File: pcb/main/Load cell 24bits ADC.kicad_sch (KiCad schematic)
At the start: 17 parts, among them J9 SJ, Q4 TRANSISTOR_PNPMMBT4403, U4 HX711

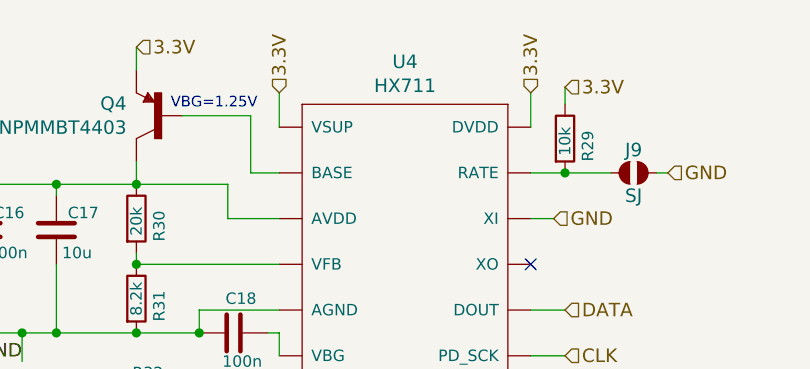
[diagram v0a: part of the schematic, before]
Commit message: fix: 3D view for HX711 and crystal
Updated route for Kicad 6.0
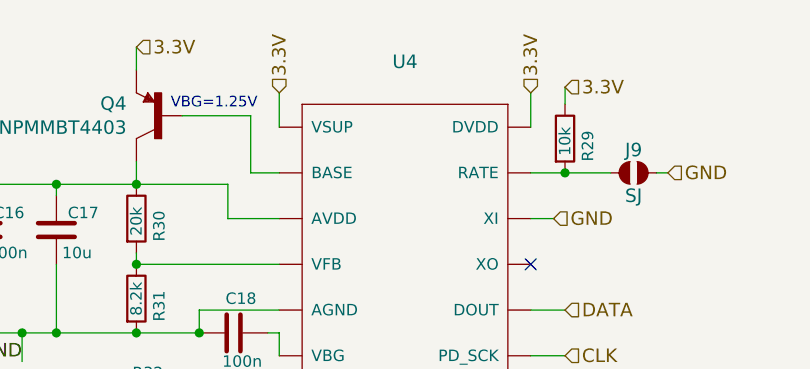
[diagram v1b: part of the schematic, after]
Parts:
- U4: value HX711 -> (none); footprint Package_SO:STC_SOP-16_3.9x9.9mm_P1.27mm -> (none)
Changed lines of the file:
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@@
       (effects (font (size 1.4986 1.4986)))
     )
-    (property "Value" "HX711" (id 1) (at 169.545 66.5226 0)
+    (property "Value" "" (id 1) (at 169.545 66.5226 0)
       (effects (font (size 1.4986 1.4986)))
     )
-    (property "Footprint" "Package_SO:STC_SOP-16_3.9x9.9mm_P1.27mm" (id 2) (at 170.815 88.9 0)
+    (property "Footprint" "" (id 2) (at 170.815 88.9 0)
       (effects (font (size 1.27 1.27)) hide)
     )

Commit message: fix: Warnings and errors in Kicad
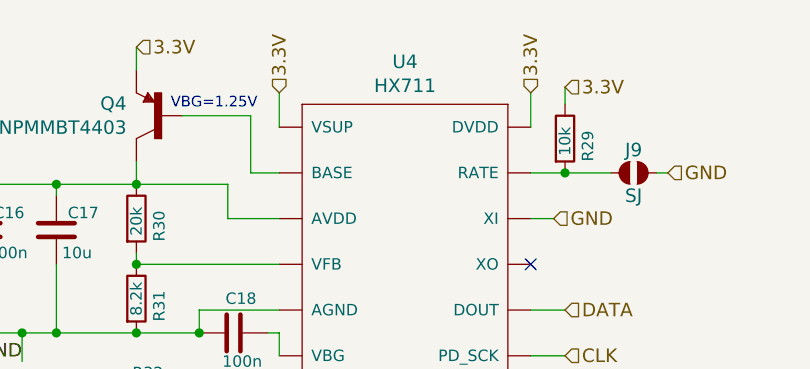
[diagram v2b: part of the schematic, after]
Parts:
- U4: value (none) -> HX711; footprint (none) -> Package_SO:STC_SOP-16_3.9x9.9mm_P1.27mm
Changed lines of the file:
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@@
       (effects (font (size 1.4986 1.4986)))
     )
-    (property "Value" "" (id 1) (at 169.545 66.5226 0)
+    (property "Value" "HX711" (id 1) (at 169.545 66.5226 0)
       (effects (font (size 1.4986 1.4986)))
     )
-    (property "Footprint" "" (id 2) (at 170.815 88.9 0)
+    (property "Footprint" "Package_SO:STC_SOP-16_3.9x9.9mm_P1.27mm" (id 2) (at 170.815 88.9 0)
       (effects (font (size 1.27 1.27)) hide)
     )
